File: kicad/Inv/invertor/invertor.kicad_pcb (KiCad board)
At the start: 2 copper layers, 24.1 x 21.3 mm, 24 parts, among them J1 Conn, J3 Conn, J4 Conn, J5 Conn, J6 Conn, Q1 IRF7343PBF, Q2 IRF7343PBF, Q3 IRLML6344

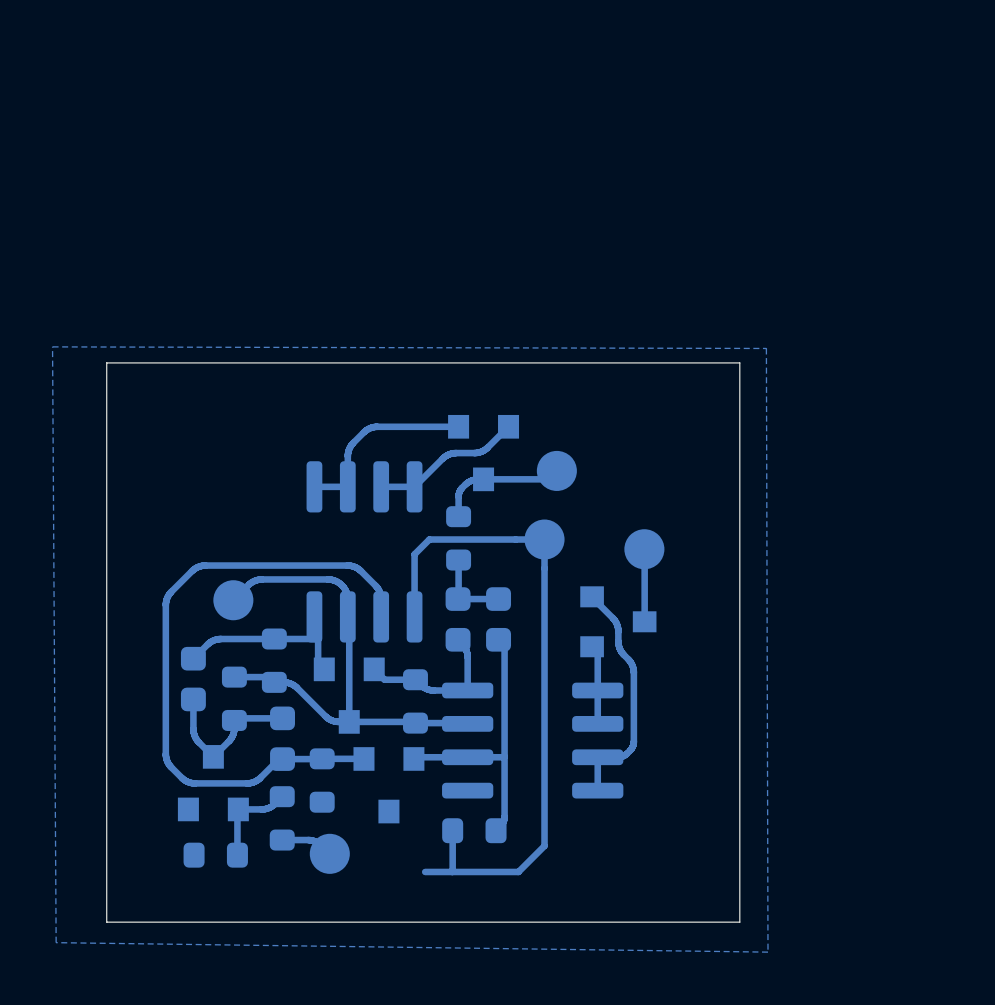
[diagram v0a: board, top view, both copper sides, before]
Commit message: изменено:      kicad/Inv/invertor/invertor-cache.lib 	изменено:      kicad/Inv/invertor/invertor.kicad_pcb 	изменено:      kicad/Inv/invertor/invertor.kicad_pcb-bak 	изменено:      kicad/Inv/invertor/invertor.sch 	изменено:      kicad/Inv/invertor/invertor.sch-bak 	изменено:      stm32cubeide/Anemometr_v3/Core/Inc/main.h 	изменено:      stm32cubeide/Anemometr_v3/Core/Src/main.c 	изменено:      stm32cubeide/Anemometr_v3/Release/Anemometr_3.bin 	изменено:      stm32cubeide/Anemometr_v3/Release/Anemometr_3.elf 	изменено:      stm32cubeide/Anemometr_v3/Release/Anemometr_3.hex 	изменено:      stm32cubeide/Anemometr_v3/Release/Anemometr_3.list 	изменено:      stm32cubeide/Anemometr_v3/Release/Core/Src/main.o 	изменено:      stm32cubeide/Anemometr_v3/Release/Core/Src/main.su
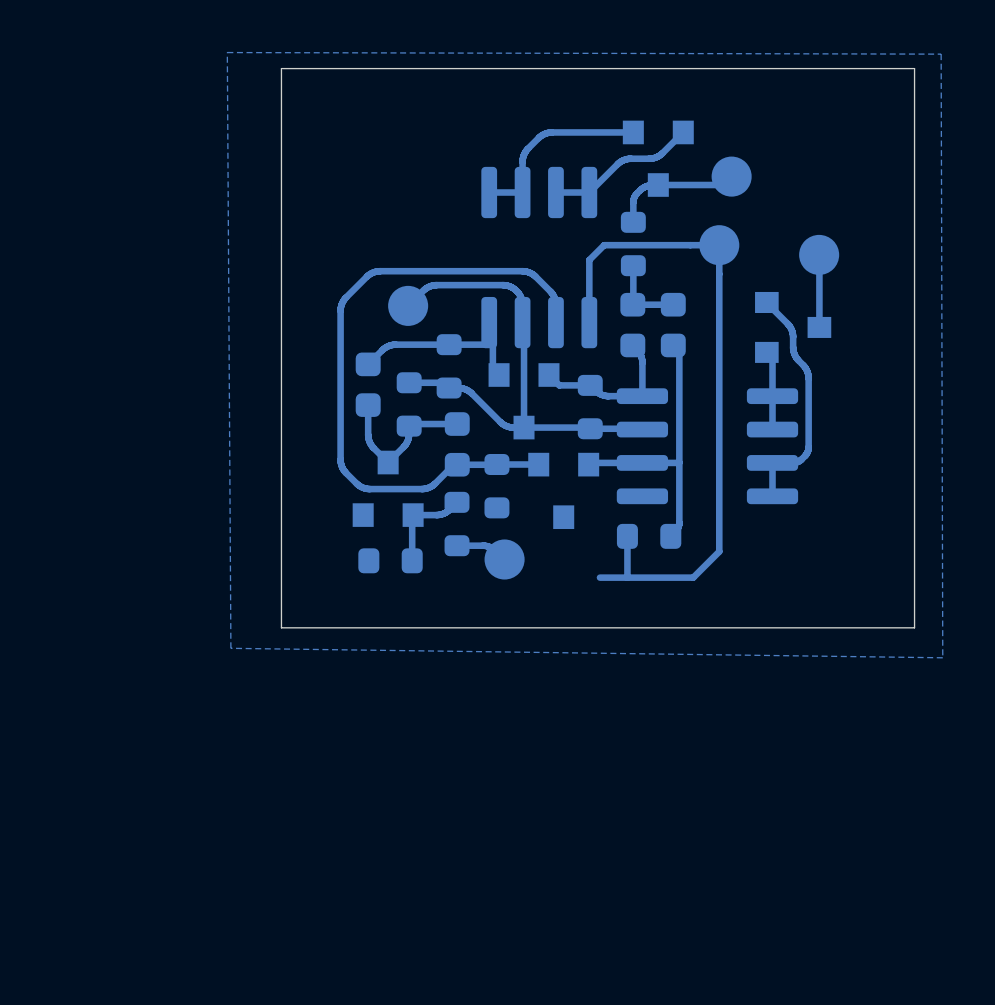
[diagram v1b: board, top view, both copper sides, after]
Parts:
- moved J1 13.0 mm to (47.6, 42.0)
- moved C1 13.0 mm to (33.8, 50.0)
- moved D1 13.0 mm to (44.8, 41.4)
- moved D4 13.0 mm to (49.9, 47.8)
- moved J4 13.0 mm to (35.3, 47.0)
- moved J6 13.0 mm to (47.1, 44.7)
- moved R2 13.0 mm to (38.7, 53.8)
- moved R3 13.0 mm to (42.2, 50.8)
- moved R7 13.0 mm to (35.3, 50.7)
- moved R8 13.0 mm to (34.6, 56.7)
- moved D3 13.0 mm to (41.2, 54.0)
- moved J3 13.0 mm to (39.0, 56.6)
- moved Q1 13.0 mm to (40.3, 45.1)
- moved R4 13.0 mm to (44.5, 55.7)
- moved Q3 13.0 mm to (34.5, 53.9)
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
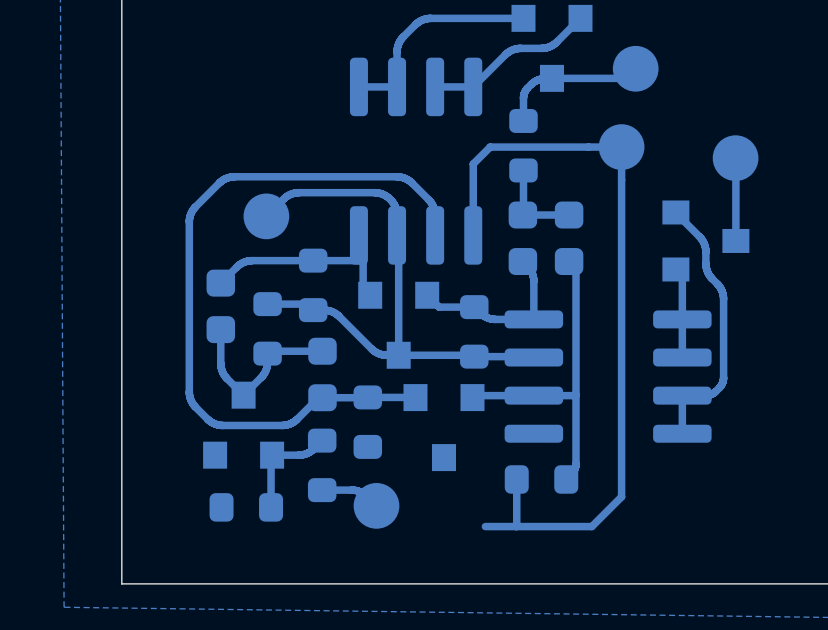
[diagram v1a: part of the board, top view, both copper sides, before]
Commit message: изменено:      kicad/Inv/invertor/invertor.kicad_pcb 	изменено:      kicad/Inv/invertor/invertor.kicad_pcb-bak 	изменено:      kicad/Inv/invertor/invertor.sch 	изменено:      kicad/Inv/invertor/invertor.sch-bak 	изменено:      stm32cubeide/Anemometr_v3/.settings/language.settings.xml 	изменено:      stm32cubeide/Anemometr_v3/Core/Inc/main.h 	изменено:      stm32cubeide/Anemometr_v3/Core/Src/main.c 	изменено:      stm32cubeide/Anemometr_v3/Core/Src/stm32f1xx_it.c 	изменено:      stm32cubeide/Anemometr_v3/Release/Anemometr_3.bin 	изменено:      stm32cubeide/Anemometr_v3/Release/Anemometr_3.elf 	изменено:      stm32cubeide/Anemometr_v3/Release/Anemometr_3.hex 	изменено:      stm32cubeide/Anemometr_v3/Release/Anemometr_3.list 	изменено:      stm32cubeide/Anemometr_v3/Release/Anemometr_3.map 	изменено:      stm32cubeide/Anemometr_v3/Release/Core/Src/main.o 	изменено:      stm32cubeide/Anemometr_v3/Release/Core/Src/main.su 	изменено:      stm32cubeide/Anemometr_v3/Release/Core/Src/stm32f1xx_it.o
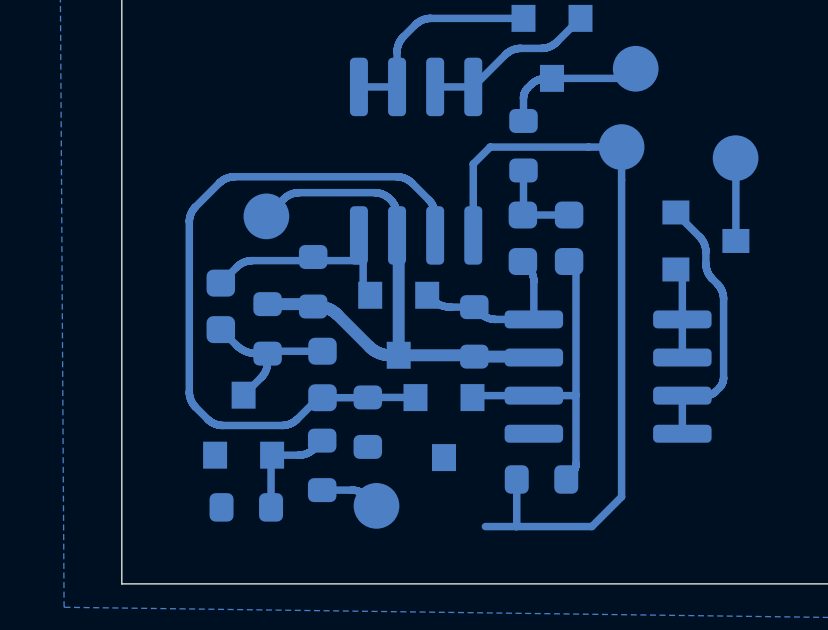
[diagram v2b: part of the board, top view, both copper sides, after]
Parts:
- moved R1 0.12 mm to (36.8, 49.1)
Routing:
- net Net-(C1-Pad2): track 6.02 -> 5.40 mm
